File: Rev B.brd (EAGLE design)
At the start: 92.1 x 61 mm, 44 parts, among them Q1 BC817-25LT1SMD

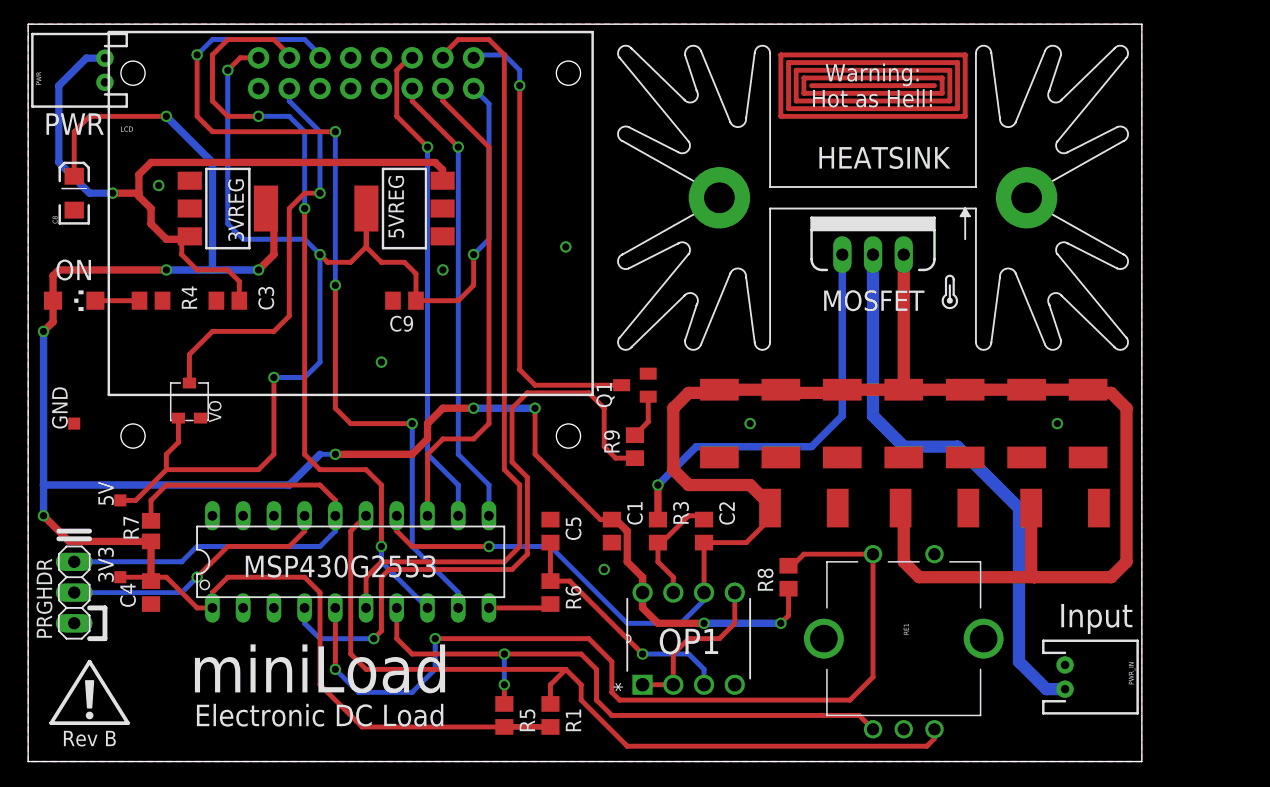
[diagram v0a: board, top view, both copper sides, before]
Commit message: Finished Rev B
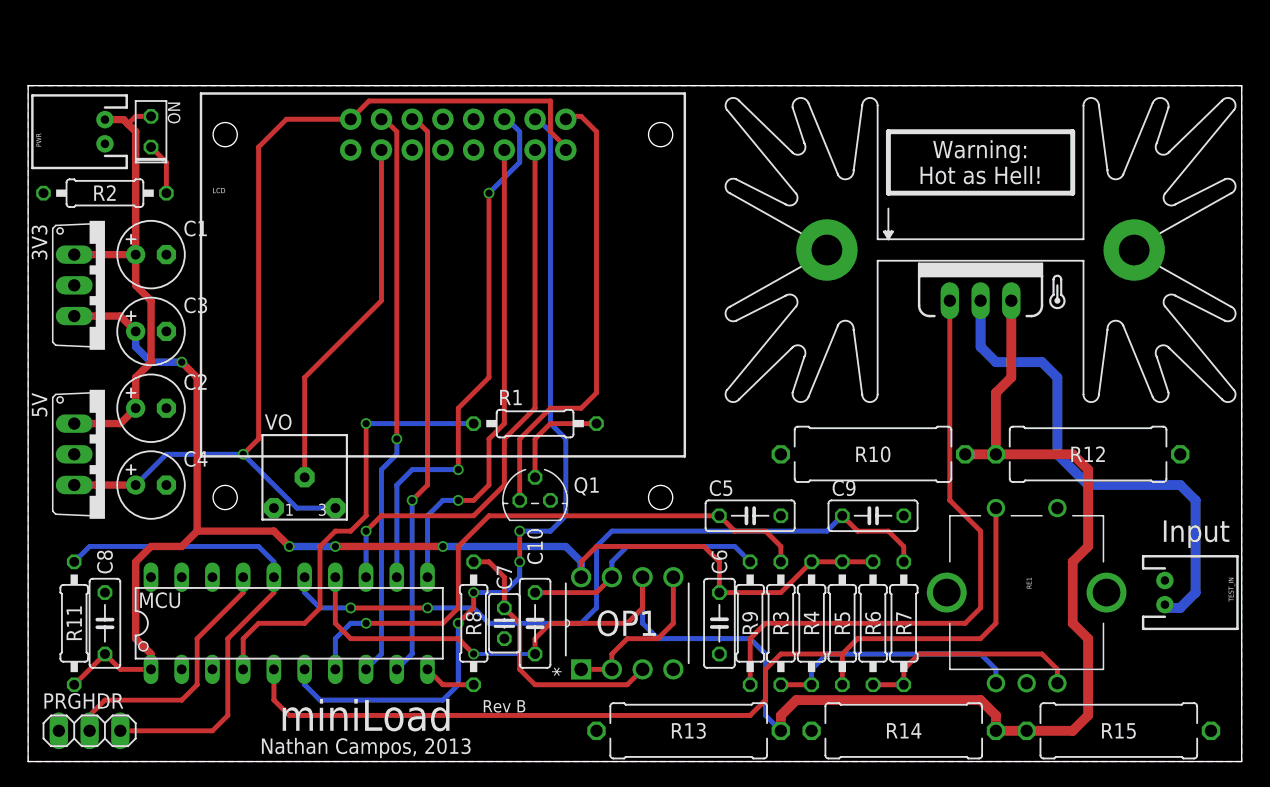
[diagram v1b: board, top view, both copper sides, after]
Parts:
- removed 3VREG: LD117AS33TR, v-reg:SOT223
- removed 5VREG: LD117AS50TR, v-reg:SOT223
- removed GND: PTR1TP10SQ, testpad:TP10SQ
- removed PWR_IN: M02JST-PTH-2, SparkFun-Connectors:JST-2-PTH
- removed R16, R17, R18: 10Ω, rcl:R2512
- removed U$2: (no value), dicons:ICON_EXL-S
- added C10: 10nF, rcl:C050-025X075
- added C6: 0.1uF, rcl:C050-025X075
- added C7: 1uF, rcl:C025-025X050
- added TEST_IN: M02JST-PTH-2, SparkFun-Connectors:JST-2-PTH
- 3V3, 5V: value PTR1TP10SQ -> 7805TV; device testpad:TP10SQ -> linear:TO220V
- C1: value 0.1uF -> 2.2uF; device rcl:C0805 -> rcl:E2,5-6
- C2: value 10nF -> 2.2uF; device rcl:C0805 -> rcl:E2,5-6
- C3: value 0.1uF -> 47uF; device rcl:C0805 -> rcl:E2,5-6
- C4: value 0.1uF -> 22uF; device rcl:C0805 -> rcl:E2,5-6
- C5: value 1uF -> 10nF; device rcl:C0805 -> rcl:C050-025X075
- C8: value 10uF -> 0.1uF; device SparkFun-Capacitors:EIA3216 -> rcl:C050-025X075
- C9: value 0.1uF -> 10nF; device rcl:C0805 -> rcl:C050-025X075
- ON: device led:CHIPLED_1206 -> led:LED2X5
- Q1: value BC817-25LT1SMD -> BC547; device transistor-npn:SOT23-BEC -> transistor-npn:TO92
- R1, R5: device rcl:R0805 -> resistor:0207/10
- R10, R12, R13, R14, R15: value 10Ω -> 5Ω; device rcl:R2512 -> rcl:P0613/15
- R11: value 10Ω -> 10kΩ; device rcl:R2512 -> resistor:0207/10
- R2: value 10Ω -> 1kΩ; device rcl:R2512 -> resistor:0207/10
- R3, R4: value 1kΩ -> 10kΩ; device rcl:R0805 -> resistor:0207/10
- R6: value 100kΩ -> 10kΩ; device rcl:R0805 -> resistor:0207/10
- R7: device resistor:R0805 -> resistor:0207/10
- R8: value 10kΩ -> 100kΩ; device rcl:R0805 -> resistor:0207/10
- R9: value 10kΩ -> 1kΩ; device rcl:R0805 -> resistor:0207/10
- VO: value TRIMPOT-2 -> 10kΩ; device SparkFun-Electromechanical:TRIMPOT_TC33 -> bourns:3362H
- moved R11 65.6 mm to (3.81, 11.4), turned to 270 degrees
- moved R7 62.7 mm to (72.4, 11.4)
- moved R4 60.8 mm to (64.8, 11.4), turned to 90 degrees
- moved R2 54.3 mm to (6.35, 47.0), turned to 0 degrees
- moved C2 46.8 mm to (10.2, 29.2), turned to 0 degrees
- moved C1 44.4 mm to (10.2, 41.9), turned to 0 degrees
- moved C9 42.6 mm to (69.8, 20.3)
- moved C8 35.7 mm to (6.35, 11.4), turned to 270 degrees
- moved R13 34.2 mm to (54.6, 2.54), turned to 0 degrees
- moved R5 29.0 mm to (67.3, 11.4), turned to 90 degrees
- moved R14 27.4 mm to (72.4, 2.54), turned to 0 degrees
- moved R6 26.8 mm to (69.8, 11.4), turned to 90 degrees
- moved R8 26.3 mm to (36.8, 11.4)
- moved R15 25.5 mm to (90.2, 2.54), turned to 180 degrees
- moved R1 24.2 mm to (41.9, 27.9), turned to 0 degrees
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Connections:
- removed net N$7: ON.C, R4.2
- new net RE_A_: R3.2, R4.1, RE1.A
- new net RE_B_: R6.1, R7.1, RE1.B
- new net VIN: 3V3.1, 5V.1, C1.+, C2.+, ON.A, PWR.2
- net +5V: now also 5V.3, C4.+, VO.3; no longer 5V.TP, 5VREG.4, C9.2, VO.1
- net BKL_CTRL: now also R1.1; no longer R9.1
- net CURR_SENSE: now also C10.2; no longer C2.2, R11.2, R16.2, R17.2, R18.2, R2.2
- net GND: now also 3V3.2, 5V.2, C1.-, C2.-, C3.-, C4.-, C5.2, C6.1, C7.2, C8.1, C9.2, Q1.1, TEST_IN.1, VO.1; no longer 3VREG.1, 5VREG.1, C1.1, C3.1, C4.1, C5.1, C8.C, C9.1, GND.TP, PWR_IN.1, Q1.E, R11.1, R16.1, R17.1, R18.1, R4.1, VO.3
- net N$16: now also Q1.2, R1.2; no longer Q1.B, R9.2
- net N$3: now also R9.2; no longer R3.2
- net N$4: now also C10.1, R9.1; no longer C2.1, R3.1
- net N$6: now also ON.K, R2.2; no longer 3VREG.3, 5VREG.3, C3.2, PWR.2
- net N$8: now also R8.2; no longer R6.2
- net N$9: now also Q1.3; no longer Q1.C
- net PWM_FILTERED: now also C7.1, R8.1; no longer C5.2, R6.1
- net RE_A: now also C5.1, R3.1; no longer R5.1, RE1.A
- net RE_B: now also C9.1, R7.2; no longer R1.1, RE1.B
- net RE_BTN: now also R5.1; no longer R8.1
- net RST: now also R11.1; no longer R7.2
- net TVIN: now also TEST_IN.2; no longer PWR_IN.2
- net VCC: now also 3V3.3, C3.+, C6.2, C8.2, R11.2, R4.2, R6.2; no longer 3V3.TP, 3VREG.4, C1.2, C4.2, C8.A, ON.A, R1.2, R7.1, R8.2
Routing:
- net VCC: track 214.9 -> 113.3 mm, vias 10 -> 4
- net N$6: track 62.8 -> 4.34 mm, vias 1 -> 0
- net N$5: track 40.6 -> 0.00 mm
- net VIN: track 0.00 -> 39.7 mm
- net N$2: track 35.6 -> 0.00 mm
- net N$12: track 30.5 -> 0.00 mm
- net LCD_EN: track 75.0 -> 47.2 mm, vias 4 -> 1
- net N$14: track 25.4 -> 0.00 mm
- net +5V: track 103.7 -> 80.7 mm, vias 4 -> 1
- net RE_A_: track 0.00 -> 21.2 mm
- net RS: track 65.9 -> 47.2 mm, vias 3 -> 1
- net RE_B_: track 0.00 -> 18.7 mm
- net CURR_SENSE: track 150.5 -> 131.8 mm
- net BKL_CTRL: track 53.1 -> 36.4 mm
- net N$3: track 33.8 -> 50.4 mm, vias 1 -> 0
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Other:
- board size 92.1 x 61 mm -> 100.3 x 55.9 mm
- board text removed: "Electronic DC Load"
- board text removed: "MOSFET"
- board text removed: "MSP430G2553"
- board text removed: "ON"
- board text removed: "PWR"
